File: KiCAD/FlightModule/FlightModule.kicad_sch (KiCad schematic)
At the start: 22 parts, among them Q1 AO3400A, Q2 AO3400A, U2 MCP2515-xST, U3 MCP2562-E-SN, U4 MB85RQ8MX, U5 MB85RQ8MX, U6 MB85RQ8MX, U7 74AHC1G14, U8 L7805

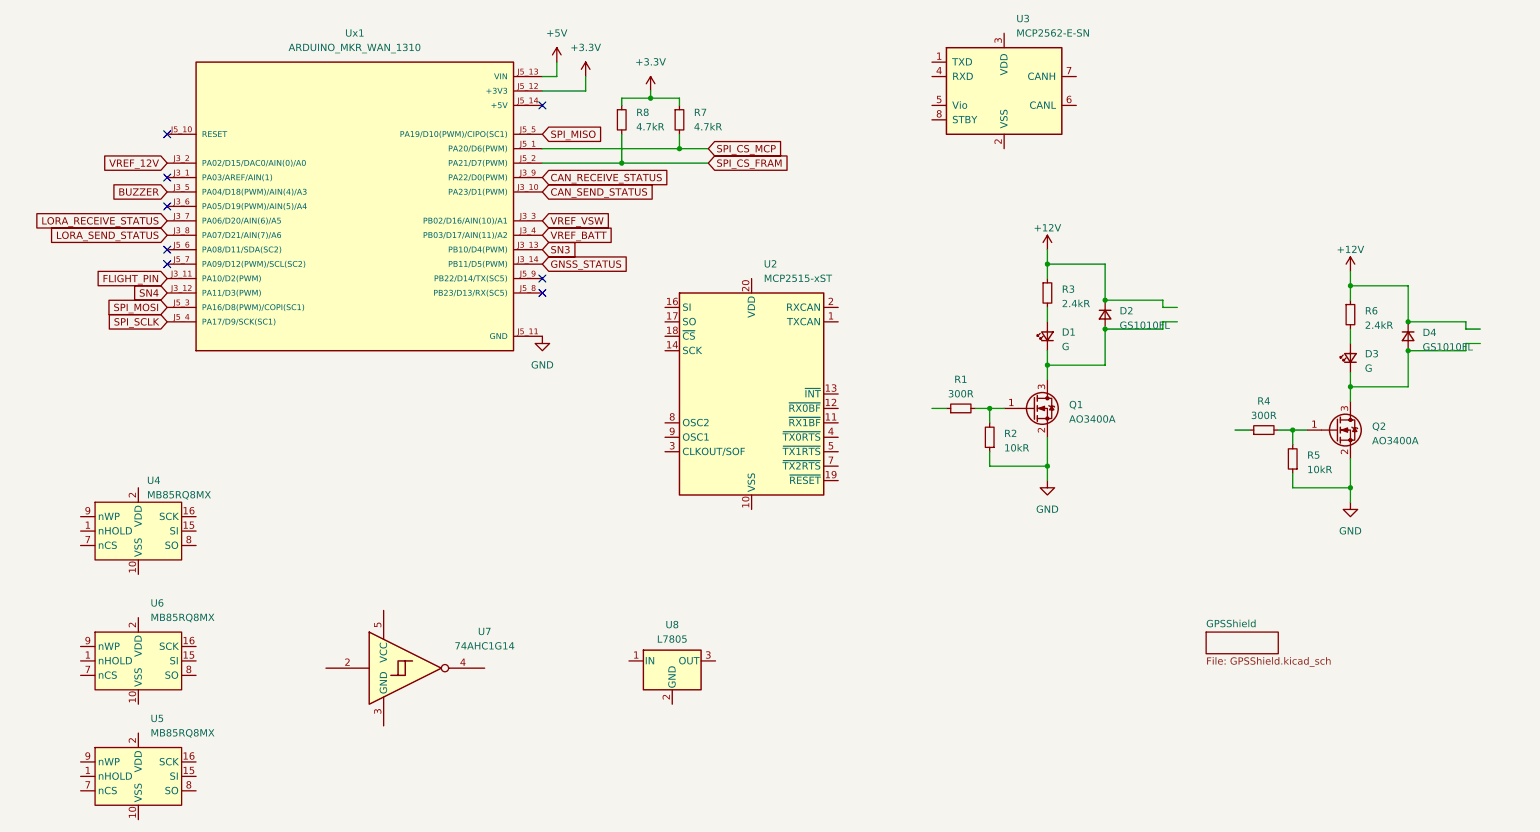
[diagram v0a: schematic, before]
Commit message: メモリ以外完成？
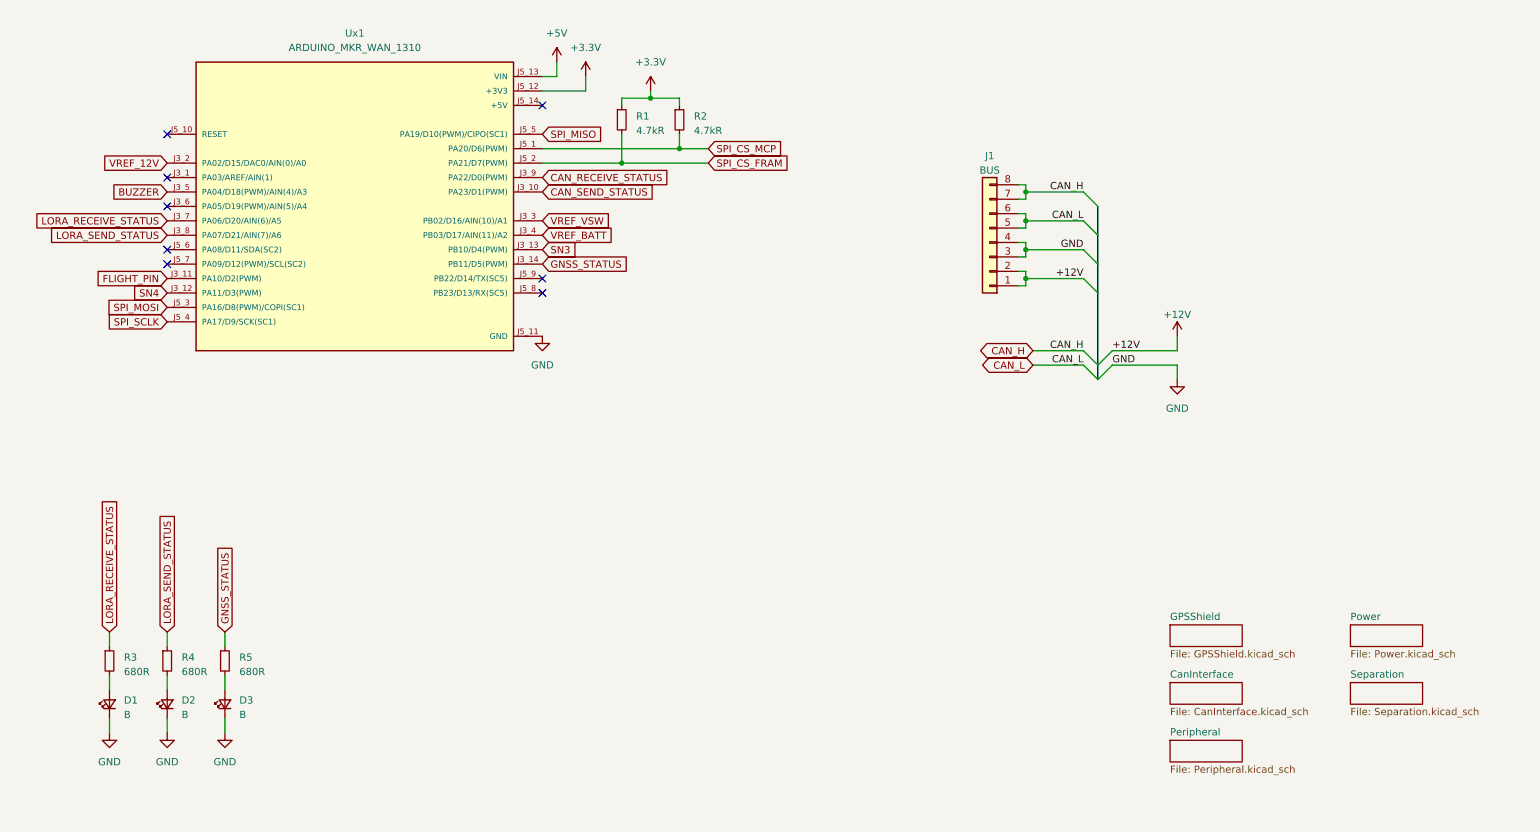
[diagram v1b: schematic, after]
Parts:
- removed D2, D4: GS1010FL, Diode_SMD:D_SOD-123F, symbol Device:D_Small
- removed Q1, Q2: AO3400A, Package_TO_SOT_SMD:SOT-23, symbol Transistor_FET:AO3400A
- removed R6: 2.4kR, Resistor_SMD:R_0603_1608Metric_Pad0.98x0.95mm_HandSolder, symbol Device:R_Small
- removed R7, R8: 4.7kR, symbol Device:R_Small
- removed U2: MCP2515-xST, Package_SO:TSSOP-20_4.4x6.5mm_P0.65mm, symbol Interface_CAN_LIN:MCP2515-xST
- removed U3: MCP2562-E-SN, Package_SO:SOIC-8_3.9x4.9mm_P1.27mm, symbol Interface_CAN_LIN:MCP2562-E-SN
- removed U4: MB85RQ8MX, Package_SO:SOIC-16W_7.5x10.3mm_P1.27mm, symbol Memory_NVRAM:MB85RQ8MX
- removed U5, U6: MB85RQ8MX, Package_SO:SOIC-16W_7.5x10.3mm_P1.27mm, symbol TSRP_IC:MB85RQ8MX
- removed U7: 74AHC1G14, symbol 74xGxx:74AHC1G14
- removed U8: L7805, symbol Regulator_Linear:L7805
- added D2: B, LED_SMD:LED_0603_1608Metric_Pad1.05x0.95mm_HandSolder, symbol Device:LED_Small
- added J1: BUS, Hirose_Connector:Hirose_DF11B-8DP-2DS, symbol Connector_Generic:Conn_01x08
- D1, D3: value G -> B
- R1: value 300R -> 4.7kR
- R2: value 10kR -> 4.7kR
- R3: value 2.4kR -> 680R
- R4: value 300R -> 680R
- R5: value 10kR -> 680R
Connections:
- net +12V: now also J1.1 (Pin_1), J1.2 (Pin_2); no longer R3.1
- net +3.3V: now also R1.1, R2.1
- net GND: now also D1.1 (K), D3.1 (K), D2.1 (K), J1.3 (Pin_3), J1.4 (Pin_4); no longer R2.1, R5.1
- net GNSS_STATUS: now also R5.1
- net LORA_RECEIVE_STATUS: now also R3.1
- net LORA_SEND_STATUS: now also R4.1
- net SPI_CS_FRAM: now also R1.2
- net SPI_CS_MCP: now also R2.2
- net at D3.2 (A): now also R5.2
- net at R4.2: now also D2.2 (A); no longer R5.2
- new net CAN_H: J1.7 (Pin_7), J1.8 (Pin_8)
- new net CAN_L: J1.5 (Pin_5), J1.6 (Pin_6)
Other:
- added sheet CanInterface (CanInterface.kicad_sch)
- added sheet Peripheral (Peripheral.kicad_sch)
- added sheet Power (Power.kicad_sch)
- added sheet Separation (Separation.kicad_sch)
